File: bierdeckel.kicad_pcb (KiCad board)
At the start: 2 copper layers, 93 x 93 mm, 58 parts, among them J1 Pogo, J2 Pogo, J3 Pogo, J4 Pogo, SW1 Address Coding, SW2 PTS526 SK15 SMTR2 LFS, SW3 PTS526 SK15 SMTR2 LFS, U1 ESP32-C3-WROOM-02, U2 BQ25176J, U3 TPS61201DRC, U4 TLV9101IDBVR

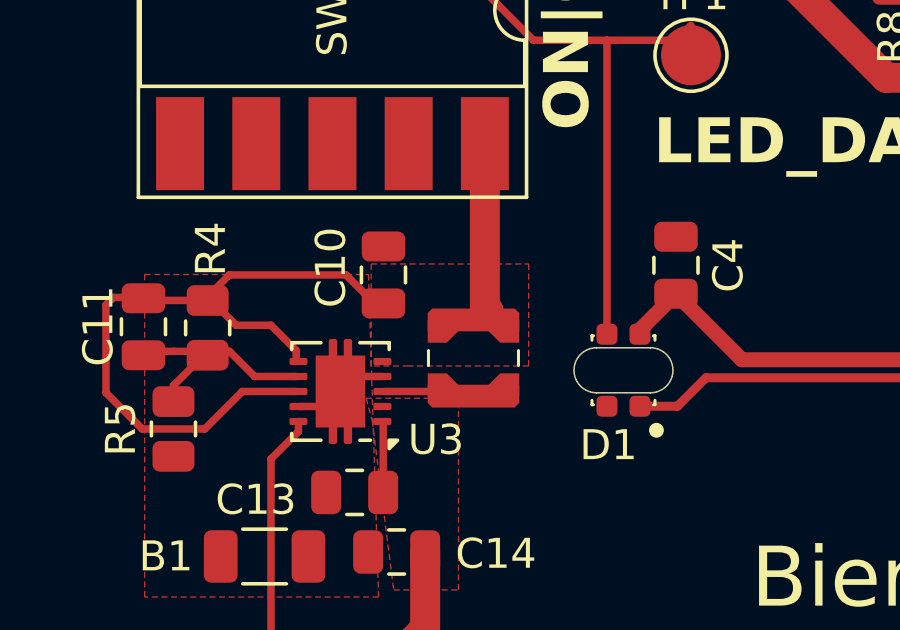
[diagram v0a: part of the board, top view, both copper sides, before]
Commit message: update design
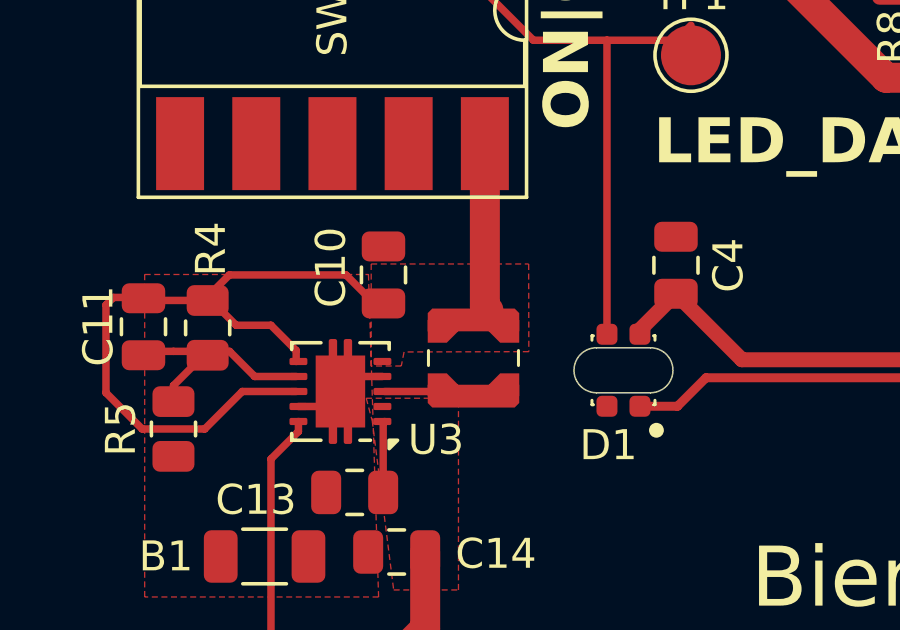
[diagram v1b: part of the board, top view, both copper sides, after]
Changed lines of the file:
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@@
 		(polygon
 			(pts
-				(xy 143.34 96.357499) (xy 139.34 96.357499) (xy 138.09 96.357499) (xy 138.09 92.957499) (xy 143.34 92.9575)
+				(xy 143.345172 95.880061) (xy 139.186213 95.889824) (xy 139.093466 96.358439) (xy 138.09 96.357499)
+				(xy 138.09 92.957499) (xy 143.34 92.9575)
 			)
 		)
